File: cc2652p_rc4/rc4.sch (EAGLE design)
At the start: 45 parts, among them IC3 CC2652R1FRGZ, Q1 SI2323DS, Q2 SI2323DS, Y1 Q22FA12800150, Y2 32.768KHz

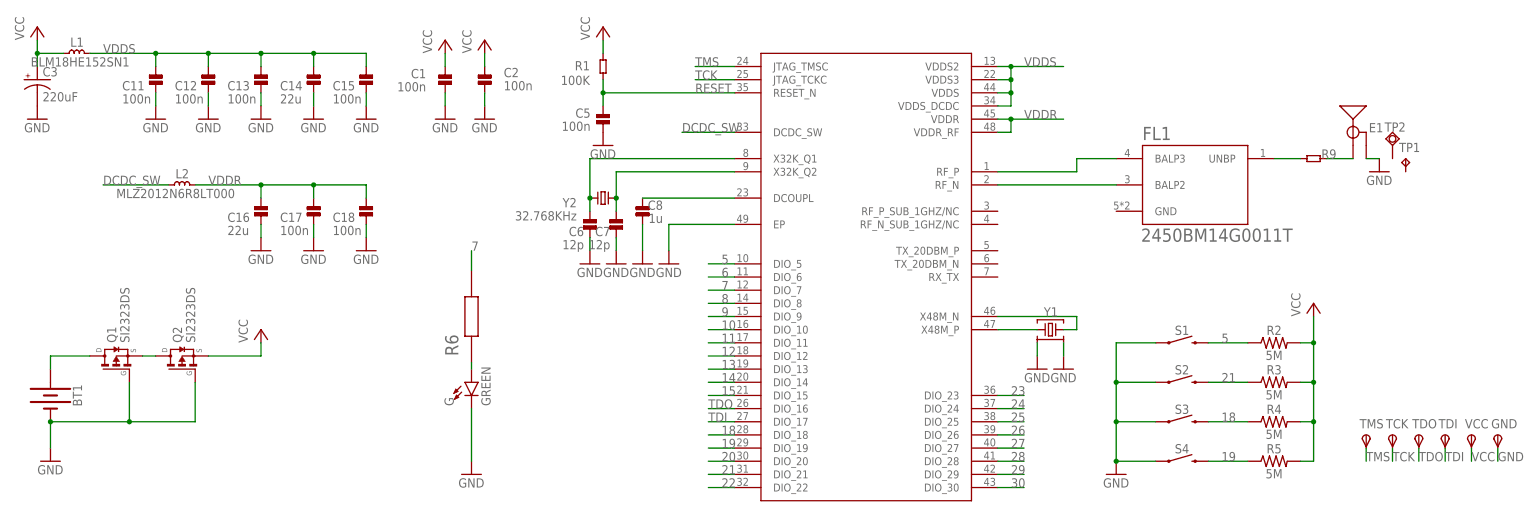
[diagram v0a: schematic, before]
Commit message: Add files via upload
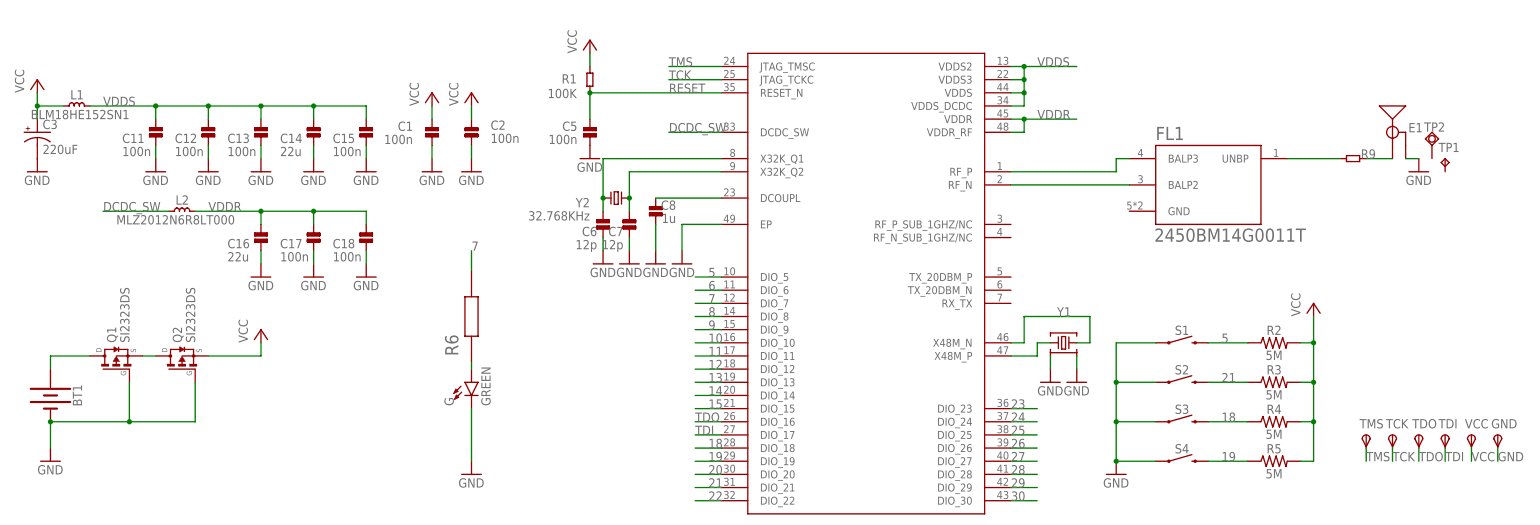
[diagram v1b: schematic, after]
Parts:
- IC3: device CC1352P1F3RGZR:CC1352P1F3RGZR -> CC2652P1FRGZR:CC2652P1FRGZRRGZ0048A-IPC_B
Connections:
- net X48M_N renamed N$4
- net X48M_P renamed N$21
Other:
- moved on the sheet: C1, C11, C12, C13, C14, C15, C16, C17, C18, C2, C3, C5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

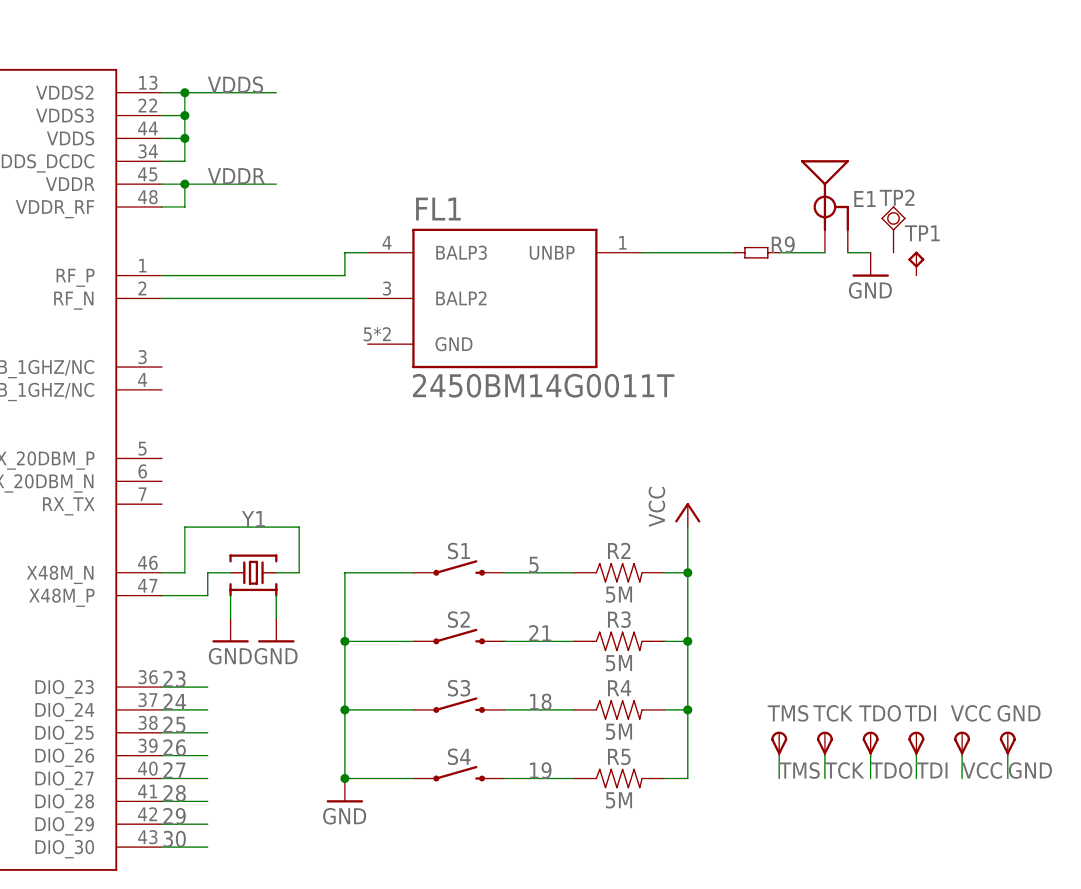
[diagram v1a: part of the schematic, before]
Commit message: Add files via upload
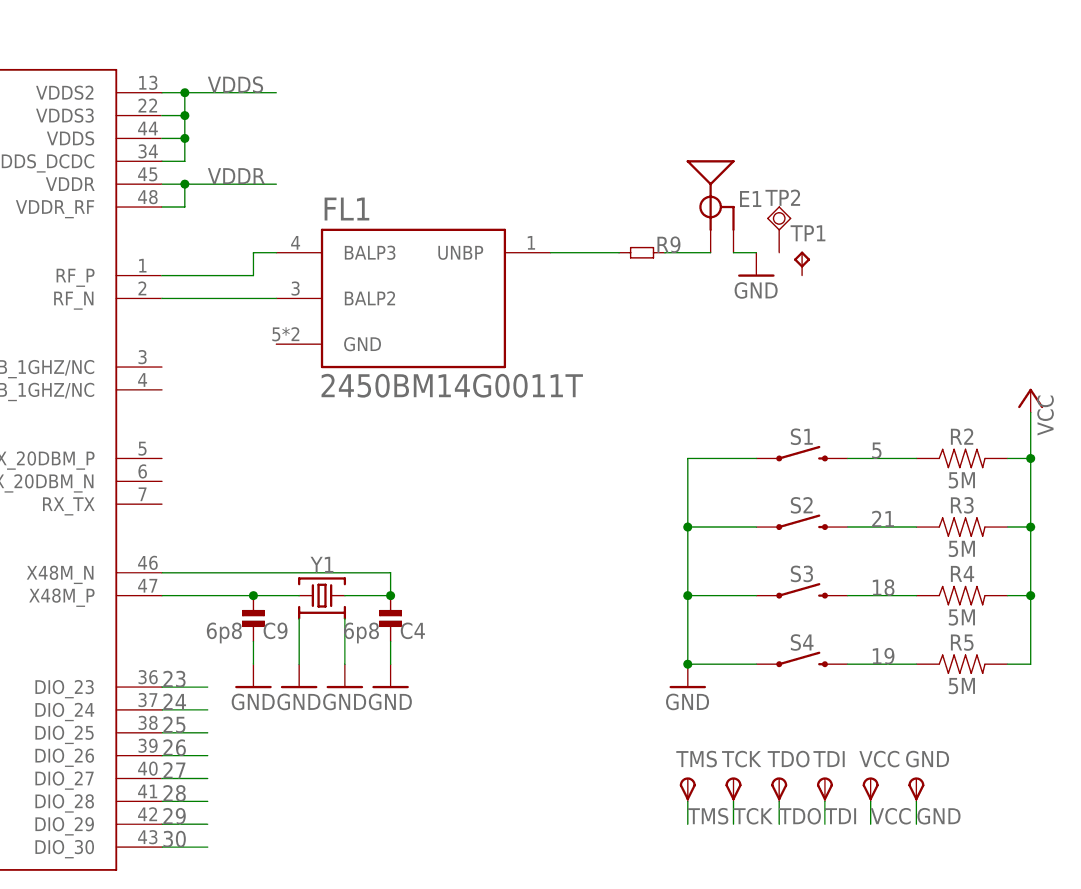
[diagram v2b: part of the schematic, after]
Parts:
- added C4, C9: 6p8, ok-discretes-dev:CAP-0402
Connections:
- net GND: now also C4.1, C9.1
- net N$21: now also C9.2
- net N$4: now also C4.2
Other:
- moved on the sheet: E1, FL1, GND, R2, R3, R4, R5, R9, S1, S2, S3, S4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
